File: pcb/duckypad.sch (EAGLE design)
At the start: 137 parts, among them IC2 REG1117, SW1 SPST_TACT-EVQQ2, SW2 SPST_TACT-EVQQ2, SW21 EC12E_SW, SW22 EC12E_SW, SW3 324_SW324_SWITCH_FOOT_HOLE, U1 USBC_16P, U2 USBC_16P, U3 ESP32-S3FN8, Y1 16MHz_12pF

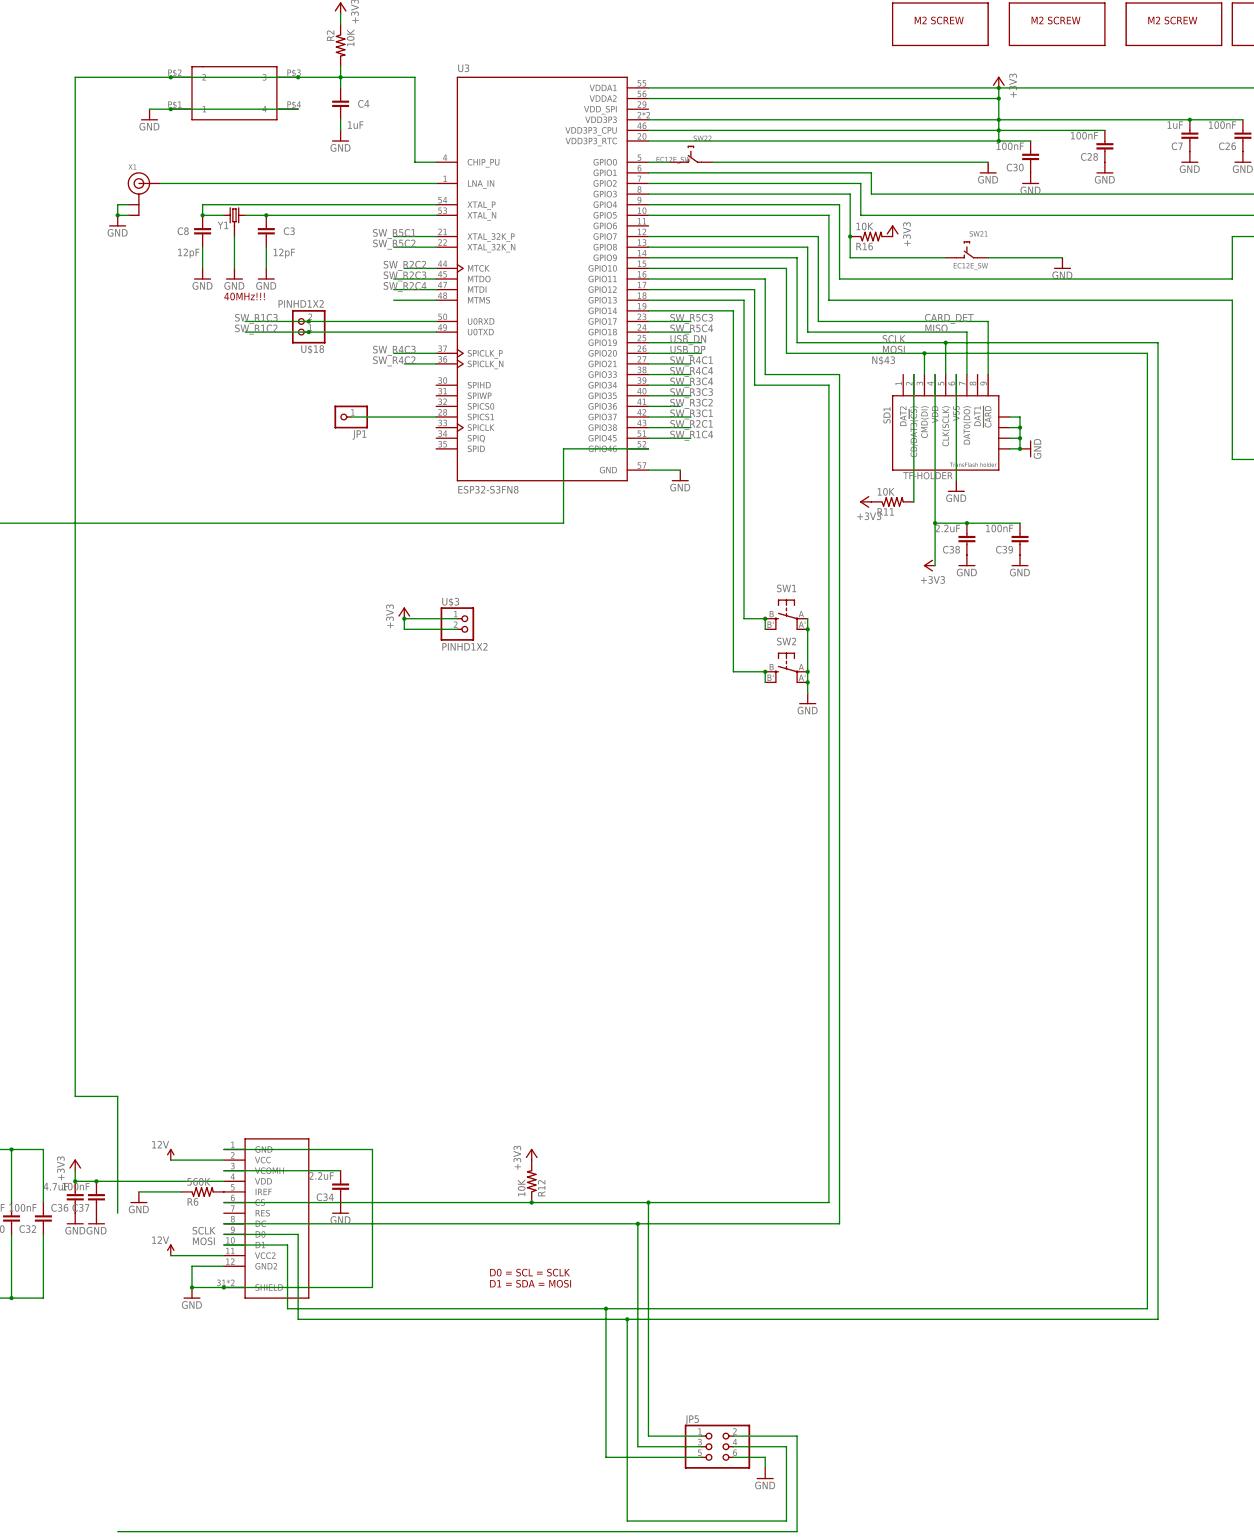
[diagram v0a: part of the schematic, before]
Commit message: updated PCB
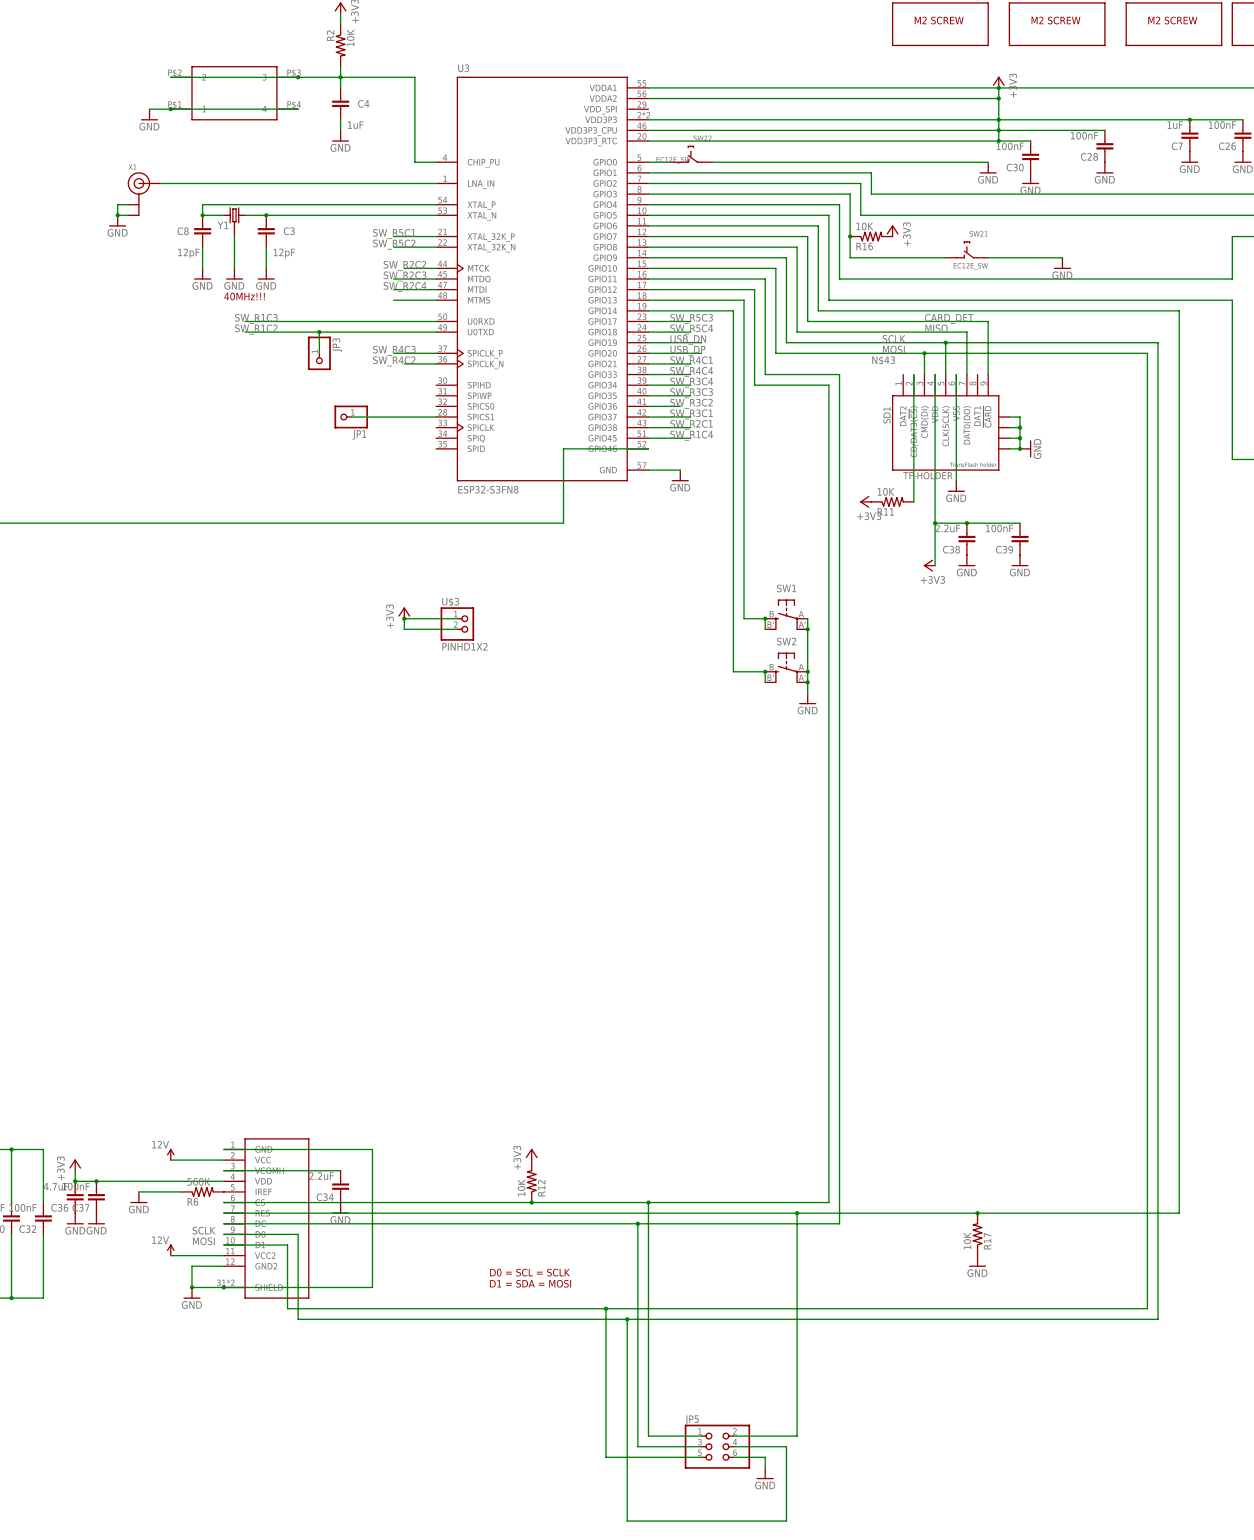
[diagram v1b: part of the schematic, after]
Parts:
- removed U$18: PINHD1X2, adafruit_changed:PINHD1X2
- added JP3: (no value), adafruit_changed:PINHD-1X1CB
- added R17: 10K, joyAnalog:RESISTOR0805-RES
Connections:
- removed net N$44: JP5.2
- new net OLED_RESET: JP5.2, R17.2, U$2.RES, U3.GPIO6
- net GND: now also R17.1
- net SW_R1C2: now also JP3.1; no longer U$18.1
- net SW_R1C3: no longer U$18.2
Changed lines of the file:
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@@
 <part name="R3" library="joyAnalog" deviceset="RESISTOR" device="0805-RES" value="5.1K"/>
 <part name="R4" library="joyAnalog" deviceset="RESISTOR" device="0805-RES" value="5.1K"/>
-<part name="U$18" library="adafruit_changed" deviceset="PINHD1X2" device=""/>
 <part name="C5" library="clock" deviceset="CAP" device="0805" value="1uF"/>
 <part name="C6" library="clock" deviceset="CAP" device="0805" value="100nF"/>
@@
 <part name="D2" library="Discrete_NOA" library_urn="urn:adsk.eagle:library:2000212" deviceset="D*" device="214AA" package3d_urn="urn:adsk.eagle:package:2068475/4" value="SS14"/>
 <part name="C46" library="clock" deviceset="CAP" device="0805" value="100nF"/>
+<part name="R17" library="joyAnalog" deviceset="RESISTOR" device="0805-RES" value="10K"/>
+<part name="GND62" library="supply1" library_urn="urn:adsk.eagle:library:371" deviceset="GND" device=""/>
+<part name="JP3" library="adafruit_changed" deviceset="PINHD-1X1" device="CB"/>
 </parts>
 <sheets>
@@
 <attribute name="VALUE" x="-1.27" y="-186.182" size="1.778" layer="96" rot="MR0"/>
 </instance>
-<instance part="U$18" gate="1" x="314.96" y="-68.58" smashed="yes" rot="R180">
-<attribute name="NAME" x="321.31" y="-74.295" size="1.778" layer="95" rot="R180"/>
-<attribute name="VALUE" x="321.31" y="-63.5" size="1.778" layer="96" rot="R180"/>
-</instance>
 <instance part="C5" gate="G$1" x="551.18" y="-15.24" smashed="yes" rot="R180">
 <attribute name="NAME" x="549.656" y="-18.161" size="1.778" layer="95" rot="R180"/>
@@
 <attribute name="NAME" x="232.156" y="-284.861" size="1.778" layer="95" rot="R180"/>
 <attribute name="VALUE" x="232.156" y="-279.781" size="1.778" layer="96" rot="R180"/>
+</instance>
+<instance part="R17" gate="G$1" x="477.52" y="-287.02" smashed="yes" rot="MR90">
+<attribute name="NAME" x="479.0186" y="-290.83" size="1.778" layer="95" rot="MR90"/>
+<attribute name="VALUE" x="474.218" y="-290.83" size="1.778" layer="96" rot="MR90"/>
+<attribute name="NAME" x="479.0186" y="-290.83" size="1.778" layer="95" rot="MR90"/>
+<attribute name="VALUE" x="474.218" y="-290.83" size="1.778" layer="96" rot="MR90"/>
+</instance>
+<instance part="GND62" gate="1" x="477.52" y="-294.64" smashed="yes">
+<attribute name="VALUE" x="474.98" y="-297.18" size="1.778" layer="96"/>
+</instance>
+<instance part="JP3" gate="G$1" x="320.04" y="-78.74" smashed="yes" rot="R270">
+<attribute name="NAME" x="323.215" y="-72.39" size="1.778" layer="95" rot="R270"/>
+<attribute name="VALUE" x="314.96" y="-72.39" size="1.778" layer="96" rot="R270"/>
 </instance>
 </instances>
@@
 <wire x1="426.72" y1="-340.36" x2="426.72" y2="-342.9" width="0.1524" layer="91"/>
 </segment>
+<segment>
+<pinref part="R17" gate="G$1" pin="1"/>
+<pinref part="GND62" gate="1" pin="GND"/>
+</segment>
 </net>
 <net name="+3V3" class="0">
@@
 <segment>
 <pinref part="U3" gate="G$1" pin="U0TXD"/>
-<pinref part="U$18" gate="1" pin="1"/>
-<wire x1="347.98" y1="-71.12" x2="317.5" y2="-71.12" width="0.1524" layer="91"/>
-<wire x1="302.26" y1="-71.12" x2="317.5" y2="-71.12" width="0.1524" layer="91"/>
-<junction x="317.5" y="-71.12"/>
+<wire x1="347.98" y1="-71.12" x2="320.04" y2="-71.12" width="0.1524" layer="91"/>
 <label x="299.72" y="-71.12" size="1.778" layer="95"/>
+<pinref part="JP3" gate="G$1" pin="1"/>
+<wire x1="320.04" y1="-71.12" x2="302.26" y2="-71.12" width="0.1524" layer="91"/>
+<wire x1="320.04" y1="-76.2" x2="320.04" y2="-71.12" width="0.1524" layer="91"/>
+<junction x="320.04" y="-71.12"/>
 </segment>
 </net>
@@
 </segment>
 <segment>
-<wire x1="317.5" y1="-68.58" x2="302.26" y2="-68.58" width="0.1524" layer="91"/>
 <pinref part="U3" gate="G$1" pin="U0RXD"/>
-<pinref part="U$18" gate="1" pin="2"/>
-<wire x1="347.98" y1="-68.58" x2="317.5" y2="-68.58" width="0.1524" layer="91"/>
-<junction x="317.5" y="-68.58"/>
+<wire x1="347.98" y1="-68.58" x2="302.26" y2="-68.58" width="0.1524" layer="91"/>
 <label x="299.72" y="-68.58" size="1.778" layer="95"/>
 </segment>
@@
 <net name="RESET" class="0">
 <segment>
-<wire x1="271.78" y1="-281.94" x2="271.78" y2="-254" width="0.1524" layer="91"/>
 <pinref part="SW3" gate="G$1" pin="2"/>
 <pinref part="SW3" gate="G$1" pin="3"/>
@@
 <wire x1="314.96" y1="-10.16" x2="325.12" y2="-10.16" width="0.1524" layer="91"/>
 <junction x="314.96" y="-10.16"/>
-<wire x1="284.48" y1="-10.16" x2="261.62" y2="-10.16" width="0.1524" layer="91"/>
-<junction x="284.48" y="-10.16"/>
-<wire x1="261.62" y1="-10.16" x2="261.62" y2="-254" width="0.1524" layer="91"/>
-<wire x1="271.78" y1="-254" x2="261.62" y2="-254" width="0.1524" layer="91"/>
 </segment>
 </net>
@@
 <net name="CARD_DET" class="0">
 <segment>
-<wire x1="439.42" y1="-48.26" x2="439.42" y2="-68.58" width="0.1524" layer="91"/>
-<wire x1="439.42" y1="-68.58" x2="480.06" y2="-68.58" width="0.1524" layer="91"/>
+<wire x1="436.88" y1="-48.26" x2="436.88" y2="-68.58" width="0.1524" layer="91"/>
+<wire x1="436.88" y1="-68.58" x2="480.06" y2="-68.58" width="0.1524" layer="91"/>
 <wire x1="480.06" y1="-68.58" x2="480.06" y2="-81.28" width="0.1524" layer="91"/>
 <pinref part="SD1" gate="G$1" pin="!CARD"/>
 <label x="464.82" y="-68.58" size="1.778" layer="95"/>
 <pinref part="U3" gate="G$1" pin="GPIO7"/>
-<wire x1="398.78" y1="-48.26" x2="439.42" y2="-48.26" width="0.1524" layer="91"/>
+<wire x1="398.78" y1="-48.26" x2="436.88" y2="-48.26" width="0.1524" layer="91"/>
 </segment>
 </net>
 <net name="MISO" class="0">
 <segment>
-<wire x1="436.88" y1="-50.8" x2="436.88" y2="-71.12" width="0.1524" layer="91"/>
-<wire x1="436.88" y1="-71.12" x2="474.98" y2="-71.12" width="0.1524" layer="91"/>
+<wire x1="434.34" y1="-50.8" x2="434.34" y2="-71.12" width="0.1524" layer="91"/>
+<wire x1="434.34" y1="-71.12" x2="474.98" y2="-71.12" width="0.1524" layer="91"/>
 <pinref part="SD1" gate="G$1" pin="DAT0(DO)"/>
 <wire x1="474.98" y1="-71.12" x2="474.98" y2="-81.28" width="0.1524" layer="91"/>
 <label x="464.82" y="-71.12" size="1.778" layer="95"/>
 <pinref part="U3" gate="G$1" pin="GPIO8"/>
-<wire x1="398.78" y1="-50.8" x2="436.88" y2="-50.8" width="0.1524" layer="91"/>
+<wire x1="398.78" y1="-50.8" x2="434.34" y2="-50.8" width="0.1524" layer="91"/>
 </segment>
 </net>
@@
 <pinref part="SD1" gate="G$1" pin="CLK(SCLK)"/>
 <wire x1="469.9" y1="-81.28" x2="469.9" y2="-73.66" width="0.1524" layer="91"/>
-<wire x1="469.9" y1="-73.66" x2="434.34" y2="-73.66" width="0.1524" layer="91"/>
-<wire x1="434.34" y1="-73.66" x2="434.34" y2="-53.34" width="0.1524" layer="91"/>
+<wire x1="469.9" y1="-73.66" x2="431.8" y2="-73.66" width="0.1524" layer="91"/>
+<wire x1="431.8" y1="-73.66" x2="431.8" y2="-53.34" width="0.1524" layer="91"/>
 <label x="454.66" y="-73.66" size="1.778" layer="95"/>
 <pinref part="U$2" gate="G$1" pin="D0"/>
@@
 <wire x1="431.8" y1="-337.82" x2="419.1" y2="-337.82" width="0.1524" layer="91"/>
 <pinref part="U3" gate="G$1" pin="GPIO9"/>
-<wire x1="398.78" y1="-53.34" x2="434.34" y2="-53.34" width="0.1524" layer="91"/>
+<wire x1="398.78" y1="-53.34" x2="431.8" y2="-53.34" width="0.1524" layer="91"/>
 </segment>
 </net>
@@
 <pinref part="SD1" gate="G$1" pin="CMD(DI)"/>
 <wire x1="464.82" y1="-81.28" x2="464.82" y2="-76.2" width="0.1524" layer="91"/>
-<wire x1="464.82" y1="-76.2" x2="431.8" y2="-76.2" width="0.1524" layer="91"/>
-<wire x1="431.8" y1="-76.2" x2="431.8" y2="-55.88" width="0.1524" layer="91"/>
+<wire x1="464.82" y1="-76.2" x2="429.26" y2="-76.2" width="0.1524" layer="91"/>
+<wire x1="429.26" y1="-76.2" x2="429.26" y2="-55.88" width="0.1524" layer="91"/>
 <label x="454.66" y="-76.2" size="1.778" layer="95"/>
 <pinref part="U$2" gate="G$1" pin="D1"/>
@@
 <junction x="388.62" y="-304.8"/>
 <pinref part="U3" gate="G$1" pin="GPIO10"/>
-<wire x1="398.78" y1="-55.88" x2="431.8" y2="-55.88" width="0.1524" layer="91"/>
+<wire x1="398.78" y1="-55.88" x2="429.26" y2="-55.88" width="0.1524" layer="91"/>
 </segment>
 </net>
@@
 </segment>
 </net>
-<net name="N$44" class="0">
+<net name="OLED_RESET" class="0">
 <segment>
 <pinref part="JP5" gate="A" pin="2"/>
 <wire x1="434.34" y1="-335.28" x2="419.1" y2="-335.28" width="0.1524" layer="91"/>
-<wire x1="271.78" y1="-358.14" x2="434.34" y2="-358.14" width="0.1524" layer="91"/>
-<wire x1="434.34" y1="-358.14" x2="434.34" y2="-335.28" width="0.1524" layer="91"/>
-</segment>
-</net>
+<pinref part="U3" gate="G$1" pin="GPIO6"/>
+<wire x1="398.78" y1="-45.72" x2="439.42" y2="-45.72" width="0.1524" layer="91"/>
+<wire x1="439.42" y1="-45.72" x2="439.42" y2="-66.04" width="0.1524" layer="91"/>
+<wire x1="439.42" y1="-66.04" x2="525.78" y2="-66.04" width="0.1524" layer="91"/>
+<pinref part="U$2" gate="G$1" pin="RES"/>
+<wire x1="525.78" y1="-66.04" x2="525.78" y2="-281.94" width="0.1524" layer="91"/>
+<wire x1="525.78" y1="-281.94" x2="477.52" y2="-281.94" width="0.1524" layer="91"/>
+<pinref part="R17" gate="G$1" pin="2"/>
+<wire x1="477.52" y1="-281.94" x2="434.34" y2="-281.94" width="0.1524" layer="91"/>
+<junction x="477.52" y="-281.94"/>
+<wire x1="434.34" y1="-281.94" x2="297.18" y2="-281.94" width="0.1524" layer="91"/>
+<wire x1="434.34" y1="-335.28" x2="434.34" y2="-281.94" width="0.1524" layer="91"/>
+<junction x="434.34" y="-281.94"/>
+</segment>
+</net>
